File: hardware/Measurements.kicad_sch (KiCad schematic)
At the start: 4 parts, among them IC1 MCP1501-10E_SN, IC6 ADA4505-1ARJZ-R7

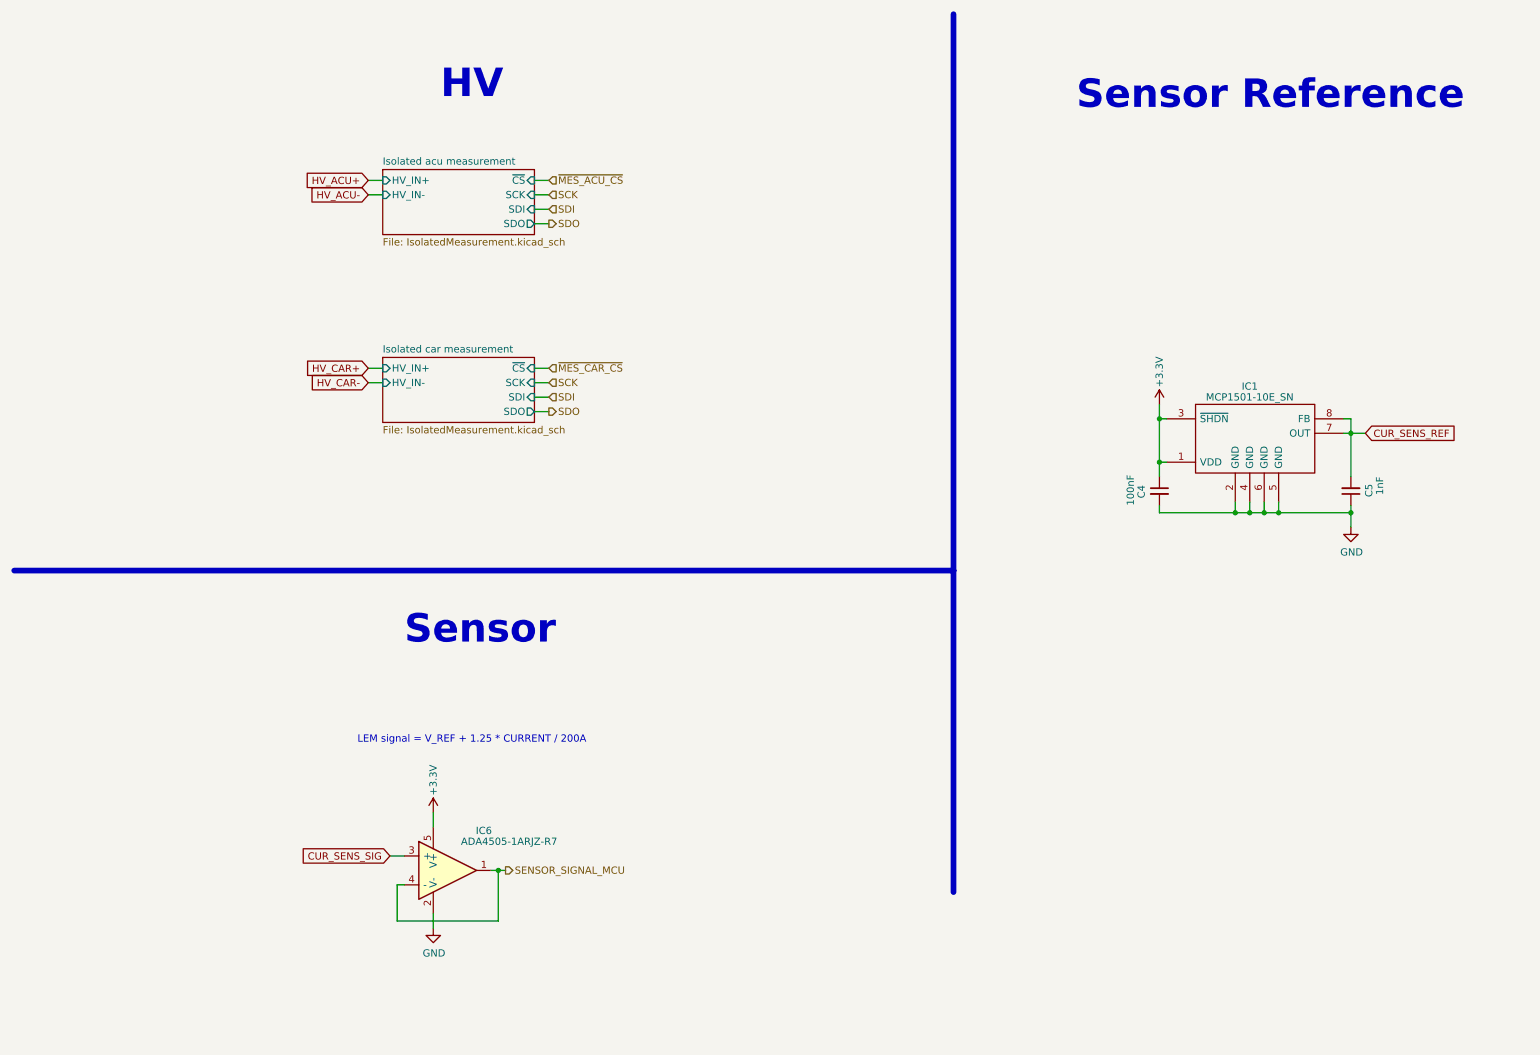
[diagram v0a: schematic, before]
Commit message: schemat sync
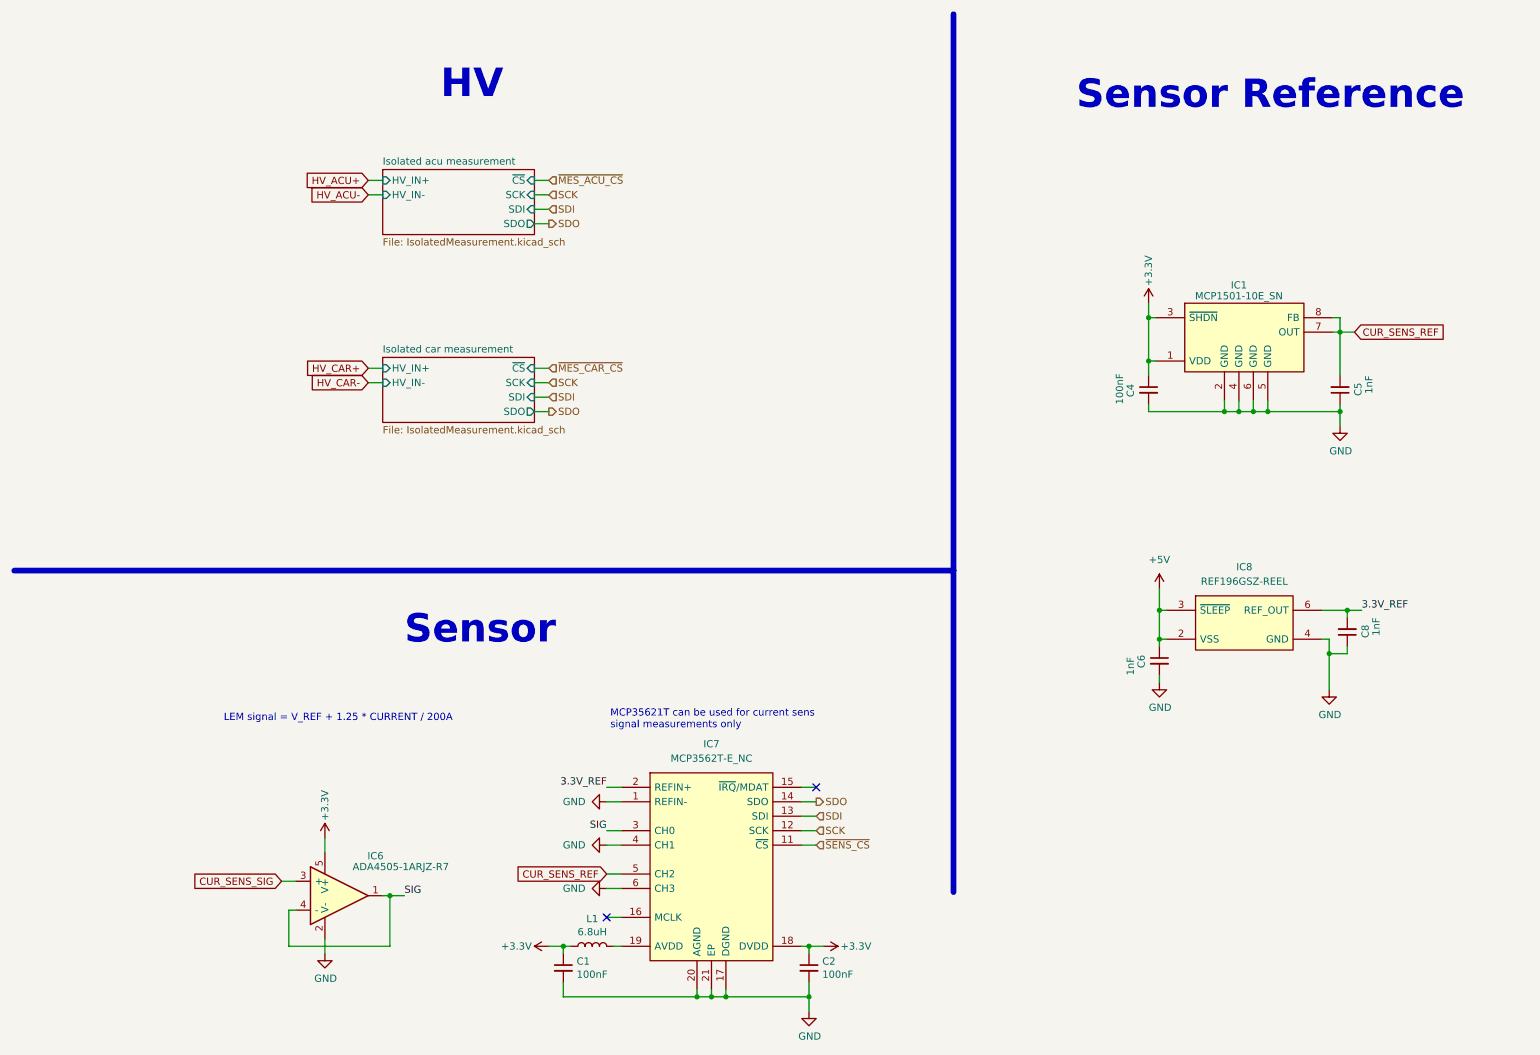
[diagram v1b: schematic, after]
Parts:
- added C1, C2: 100nF, Capacitor_SMD:C_0603_1608Metric, symbol Device:C_Small
- added C6, C8: 1nF, Capacitor_SMD:C_0603_1608Metric, symbol Device:C_Small
- added IC7: MCP3562T-E_NC, QFN40P300X300X60-21N-D, symbol MCP3562T-E_NC:MCP3562T-E_NC
- added IC8: REF196GSZ-REEL, SOIC127P600X175-8N, symbol REF196GSZ-REEL:REF196GSZ-REEL
- added L1: 6.8uH, Inductor_SMD:L_1206_3216Metric, symbol Device:L
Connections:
- net SENSOR_SIGNAL_MCU is gone; now on net SIG: IC6.1, IC6.4 (-)
- net +3V3: now also C1.1, C2.1, IC7.18 (DVDD), L1.1
- net CUR_SENS_REF: now also IC7.5 (CH2)
- net GND: now also C1.2, C2.2, C6.2, C8.1, IC7.1 (REFIN-), IC7.17 (DGND), IC7.20 (AGND), IC7.21 (EP), IC7.4 (CH1), IC7.6 (CH3), IC8.4 (GND)
- net SCK: now also IC7.12 (SCK)
- net SDI: now also IC7.13 (SDI)
- net SDO: now also IC7.14 (SDO)
- net SIG: now reaches IC6.1
- net SIG: now also IC7.3 (CH0)
- new net: IC7.19 (AVDD), L1.2
- new net +5V: C6.1, IC8.2 (VSS), IC8.3 (~{SLEEP})
- new net 3.3V_REF: C8.2, IC7.2 (REFIN+), IC8.6 (REF_OUT)
- new net ~{SENS_CS}: IC7.11 (~{CS})
- no-connect marks 0 -> 2
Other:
- note added: "MCP35621T can be used for current sens signal measurements only"
- moved on the sheet: C4, C5, IC6
